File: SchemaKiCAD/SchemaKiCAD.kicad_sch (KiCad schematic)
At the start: 19 parts, among them J1 Connettore per PLC, M1 ASSE X, M2 ASSE Y, M3 ASSE Z, Q1 MOSFET

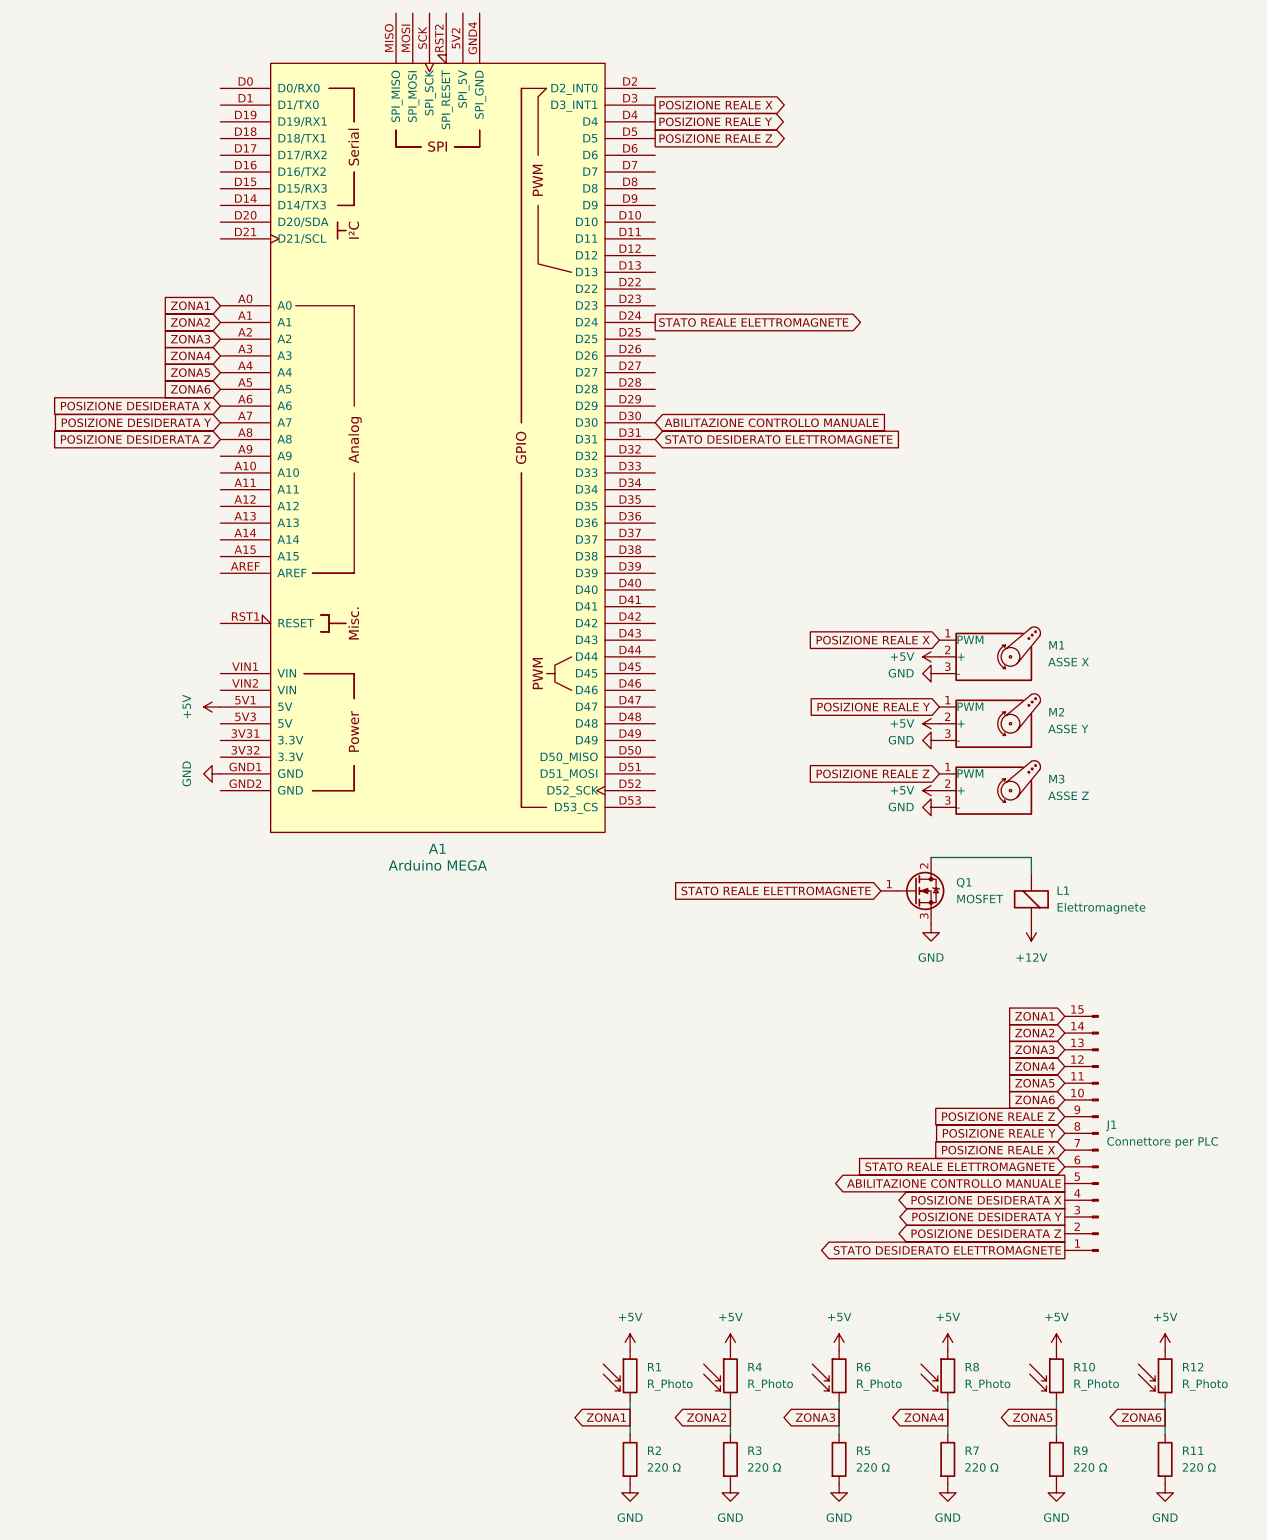
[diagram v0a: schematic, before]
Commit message: feat: sperabilmente tuttapposto!
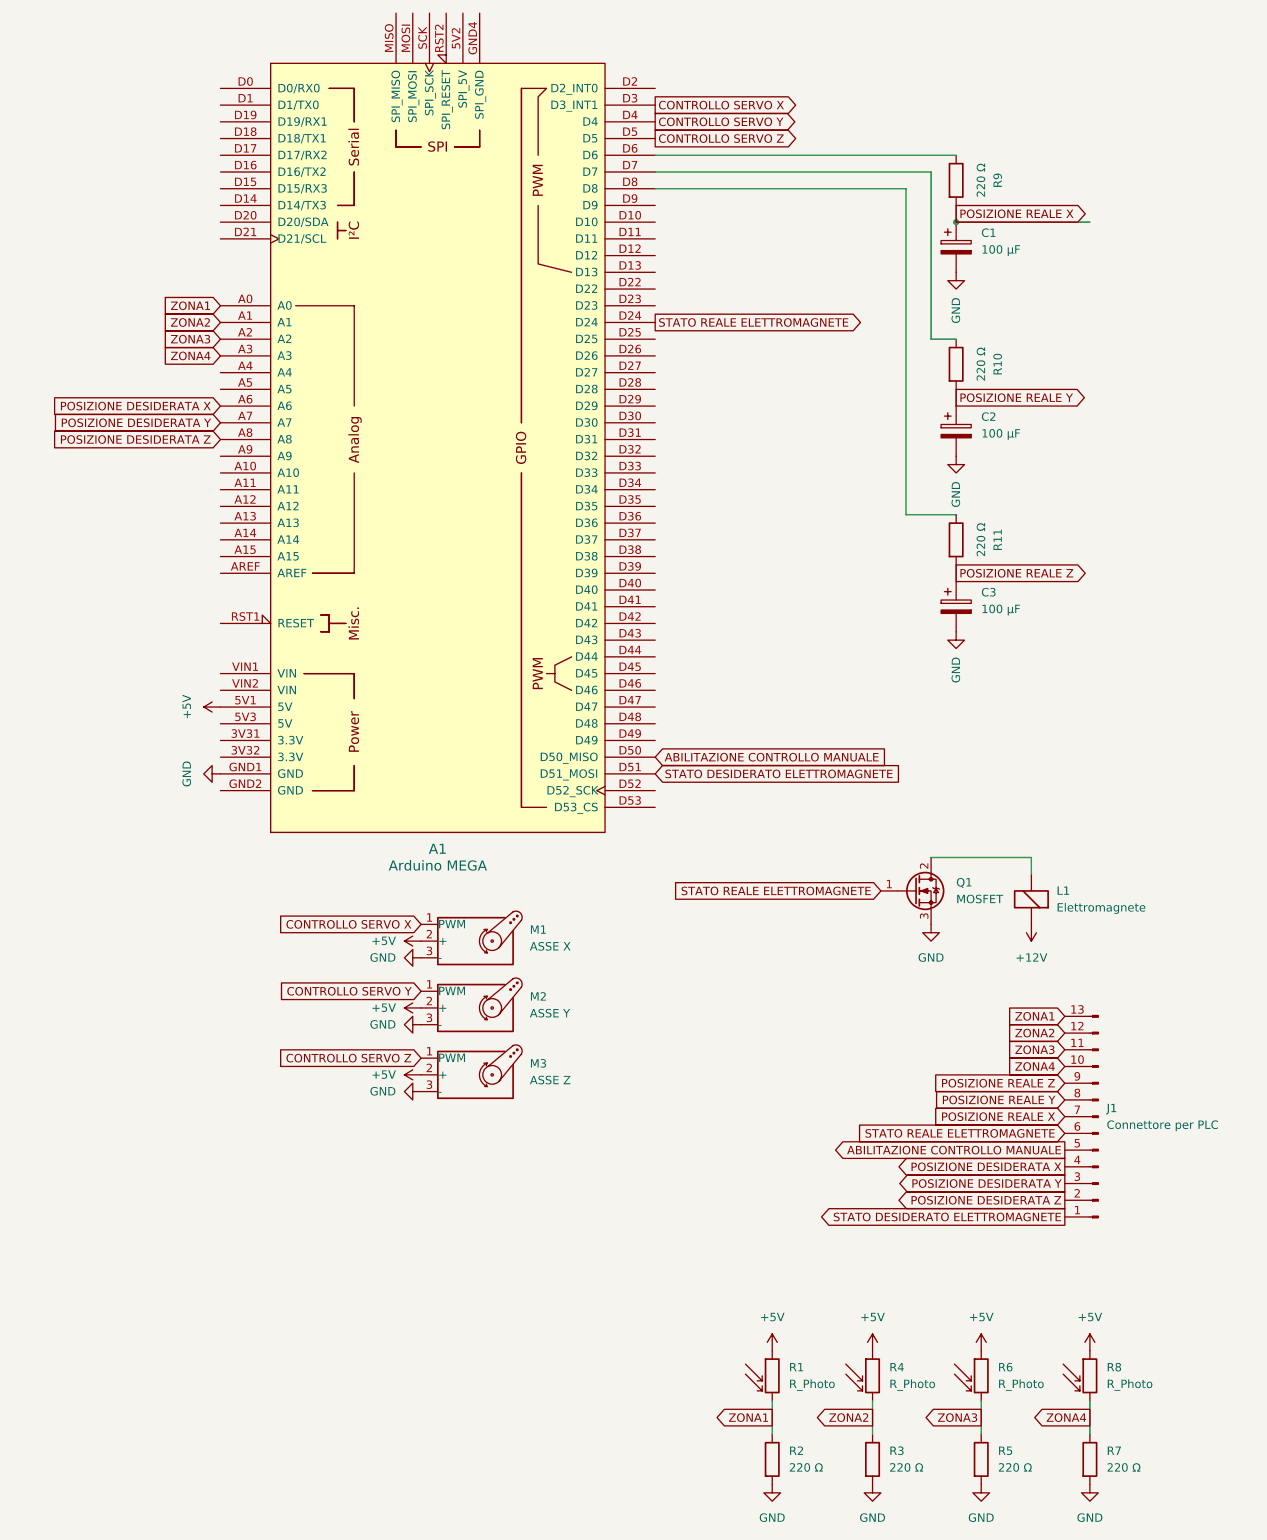
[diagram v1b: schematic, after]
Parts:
- removed J1: Connettore per PLC, symbol Connector:Conn_01x15_Pin
- removed R10, R12: R_Photo, symbol Device:R_Photo
- added C1, C2, C3: 100 µF, symbol Device:C_Polarized
- added J1: Connettore per PLC, symbol Connector:Conn_01x13_Pin
- added R10: 220 Ω, symbol Device:R
- R11, R9: value 220 Ω -> 220 Ω
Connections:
- net ABILITAZIONE CONTROLLO MANUALE: now also A1.D50 (D50_MISO), J1.5 (Pin_5); no longer A1.D30
- net GND: now also C1.2, C2.2, C3.2; no longer R11.2, R9.2
- net POSIZIONE DESIDERATA X: now also J1.4 (Pin_4)
- net POSIZIONE DESIDERATA Y: now also J1.3 (Pin_3)
- net POSIZIONE DESIDERATA Z: now also J1.2 (Pin_2)
- net POSIZIONE REALE X: now also R9.2, C1.1, J1.7 (Pin_7); no longer A1.D3 (D3_INT1), M1.1 (PWM)
- net POSIZIONE REALE Y: now also C2.1, J1.8 (Pin_8), R10.2; no longer A1.D4, M2.1 (PWM)
- net POSIZIONE REALE Z: now also R11.2, C3.1, J1.9 (Pin_9); no longer A1.D5, M3.1 (PWM)
- net STATO DESIDERATO ELETTROMAGNETE: now also A1.D51 (D51_MOSI), J1.1 (Pin_1); no longer A1.D31
- net STATO REALE ELETTROMAGNETE: now also J1.6 (Pin_6)
- net ZONA1: now also J1.13 (Pin_13)
- net ZONA2: now also J1.12 (Pin_12)
- net ZONA3: now also J1.11 (Pin_11)
- net ZONA4: now also J1.10 (Pin_10)
- net at A1.D6: now also R9.1
- net at A1.D7: now also R10.1
- net at A1.D8: now also R11.1
- net ZONA5: no longer names the net of A1.A4
- net ZONA5: no longer R9.1
- net ZONA6: no longer names the net of A1.A5
- net ZONA6: no longer R11.1
- new net CONTROLLO SERVO X: A1.D3 (D3_INT1), M1.1 (PWM)
- new net CONTROLLO SERVO Y: A1.D4, M2.1 (PWM)
- new net CONTROLLO SERVO Z: A1.D5, M3.1 (PWM)
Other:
- moved on the sheet: M1, M2, M3, R1, R2, R3, R4, R5, R6, R7, R8
